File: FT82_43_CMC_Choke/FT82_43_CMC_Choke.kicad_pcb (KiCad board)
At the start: 2 copper layers, 73 x 25 mm, 15 parts, among them J1 Conn_01x01_Pin, J4 Conn_01x01_Pin, J6 Conn_01x01_Pin

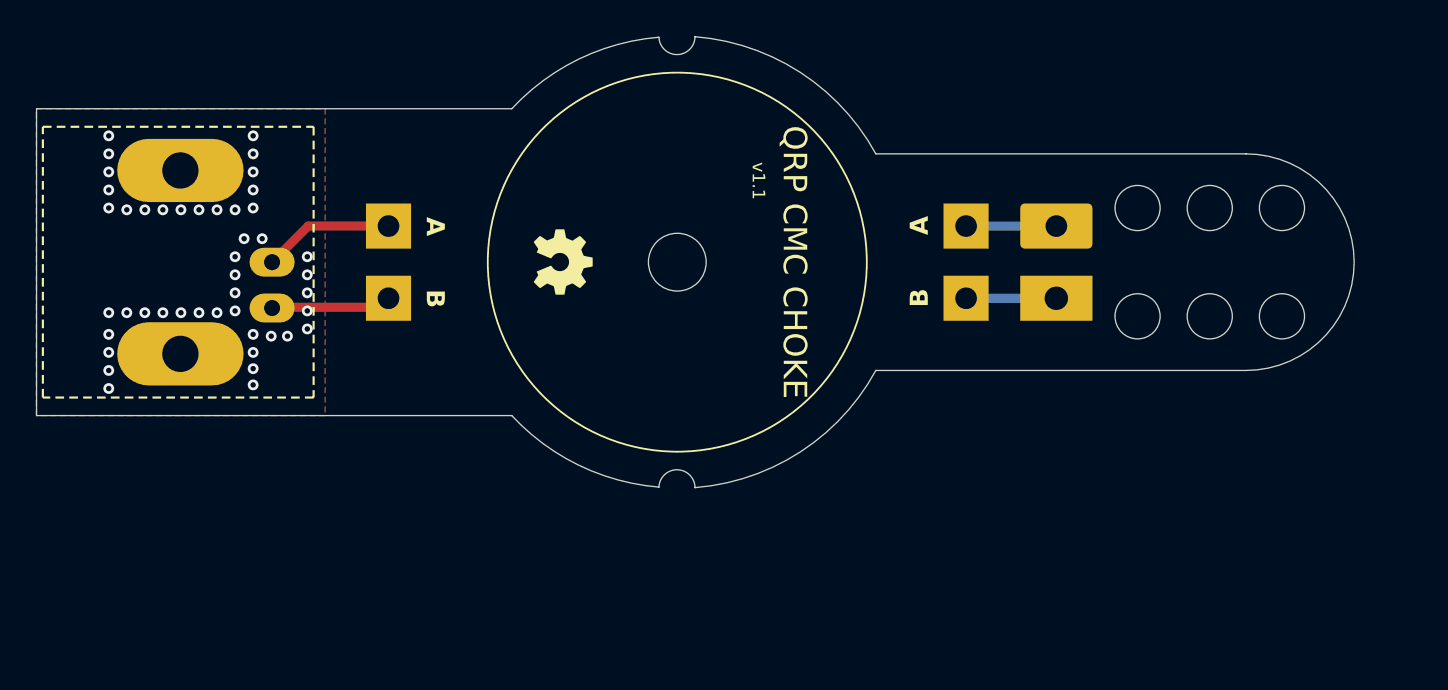
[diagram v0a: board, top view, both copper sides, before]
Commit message: Update docs
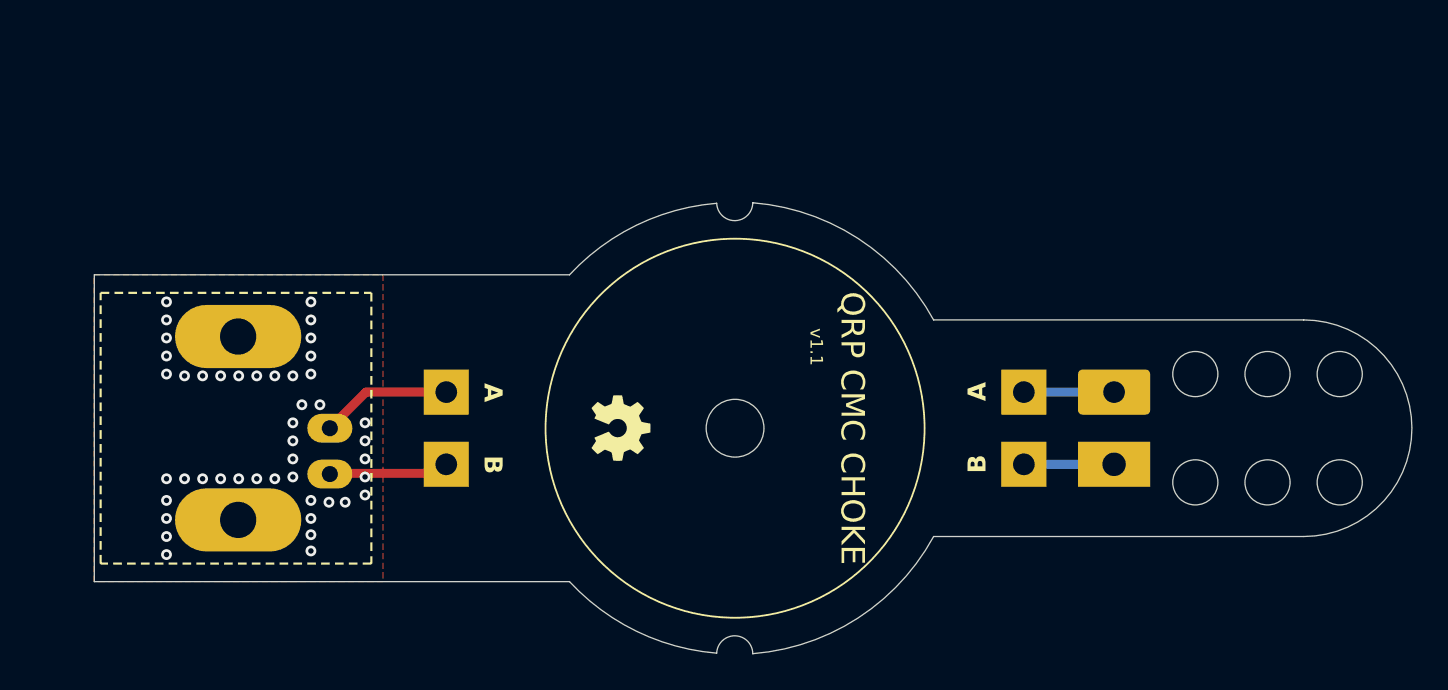
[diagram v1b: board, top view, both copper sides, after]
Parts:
- moved C1 9.74 mm to (127.8, 100.2)
- moved ? 9.74 mm to (175.7, 97.2)
- moved ? 9.74 mm to (183.7, 103.2)
- moved ? 9.74 mm to (179.7, 103.2)
- moved ? 9.74 mm to (175.7, 103.2)
- moved ? 9.74 mm to (183.7, 97.2)
- moved ? 9.74 mm to (179.7, 97.2)
- moved COAX1 9.74 mm to (171.2, 102.2)
- moved F1 9.74 mm to (134.2, 102.2)
- moved F2 9.74 mm to (166.2, 98.2)
- moved J1 9.74 mm to (134.2, 98.2)
- moved J4 9.74 mm to (166.2, 102.2)
- moved J6 9.74 mm to (171.2, 98.2)
- moved REF** 9.74 mm to (150.2, 100.2)
- moved REF** 9.74 mm to (142.8, 100.1)
